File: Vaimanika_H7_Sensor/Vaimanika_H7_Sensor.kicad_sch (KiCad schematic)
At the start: 71 parts, among them SW1 TS-1088-AR02016, U1 TCAN334G, U2 STM32H743VITx, U3 NCP163ASN330T1G, U4 MS5611-01BA, U5 ICM-42688-P, U6 ICM-42688-P, U7 W25Q128JVS, U8 RT9080-33GJ5, U9 BMI088, Y1 25 MHz

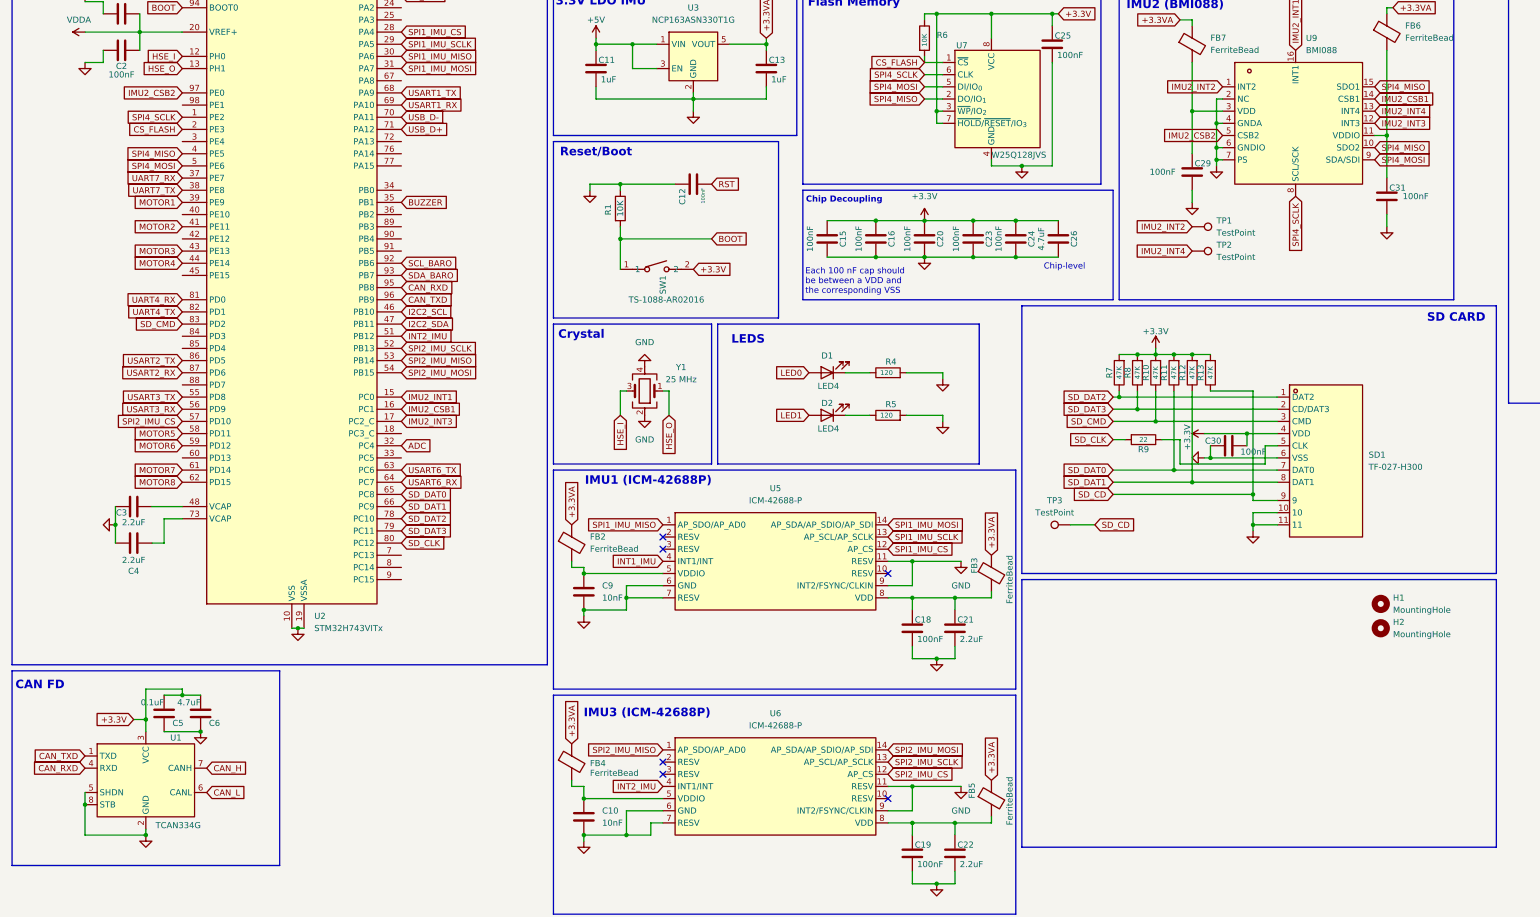
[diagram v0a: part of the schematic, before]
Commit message: 20-05-2026
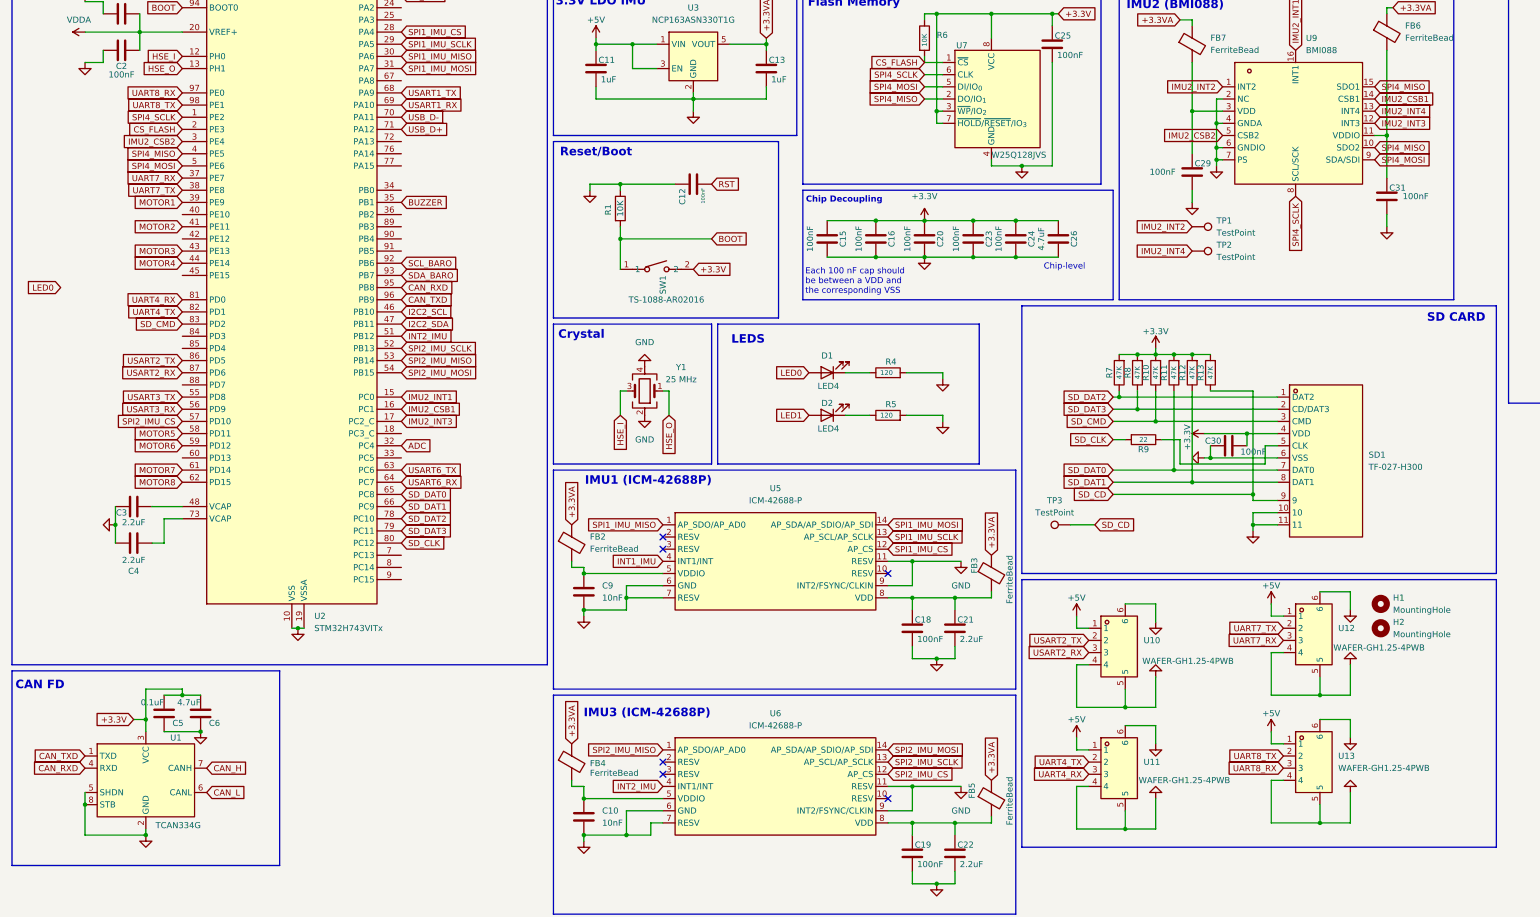
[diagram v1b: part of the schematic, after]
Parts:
- added U10, U11, U12, U13: WAFER-GH1.25-4PWB, New_Library:CONN-SMD_4P-P1.25_XUNPU_WAFER-GH1.25-4PWB, symbol New_Library:WAFER-GH1.25-4PWB
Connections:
- net +5V: now also U10.1, U11.1, U12.1, U13.1
- net GND: now also U10.4, U10.5, U10.6, U11.4, U11.5, U11.6, U12.4, U12.5, U12.6, U13.4, U13.5, U13.6
- net IMU2_CSB2: now also U2.3 (PE4); no longer U2.97 (PE0)
- net UART4_RX: now also U11.3
- net UART4_TX: now also U11.2
- net UART7_RX: now also U12.3
- net UART7_TX: now also U12.2
- net USART2_RX: now also U10.3
- net USART2_TX: now also U10.2
- net UART8_TX: now reaches U2.98 (PE1)
- net UART8_TX: now also U13.2
- new net UART8_RX: U13.3, U2.97 (PE0)
